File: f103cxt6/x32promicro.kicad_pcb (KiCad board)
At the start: 2 copper layers, 17.8 x 33 mm, 24 parts, among them J1 USB2.0_C_v3, J2 ProMicro-LeftPin-NoGND, J3 ProMicro-RightPin, J4 SWD-MCU_Side-10Pin, SW2 SW_Push, U1 AMS1117-3.3, U2 STM32V103C8T6, Y1 8M

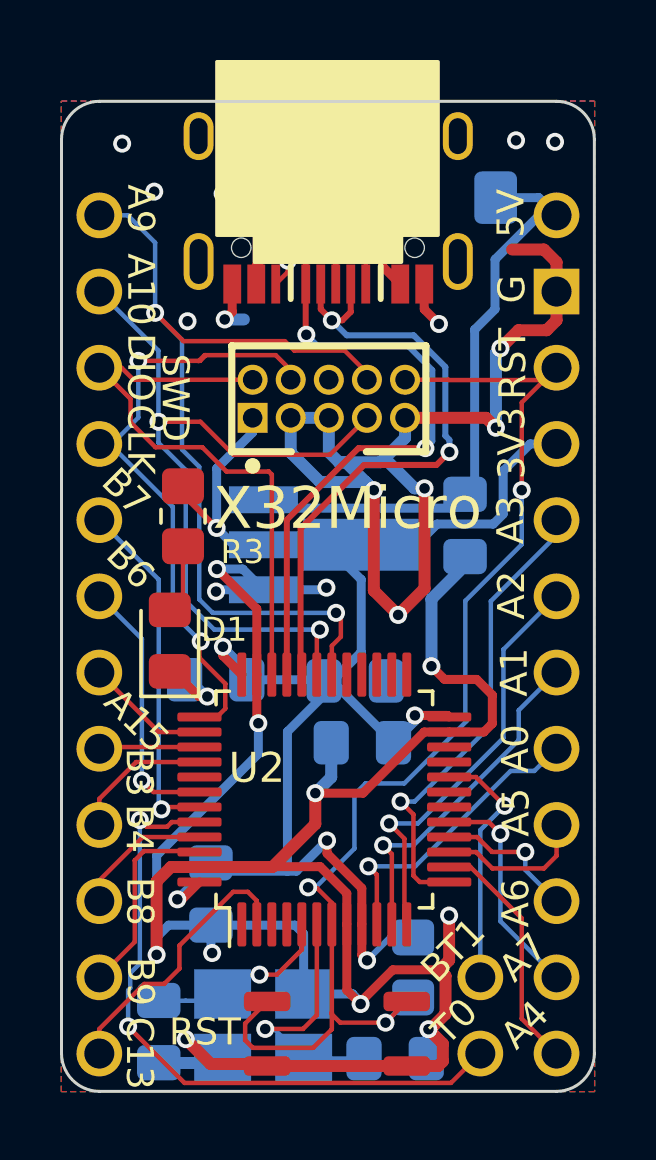
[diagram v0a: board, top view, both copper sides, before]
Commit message: v1.2.0
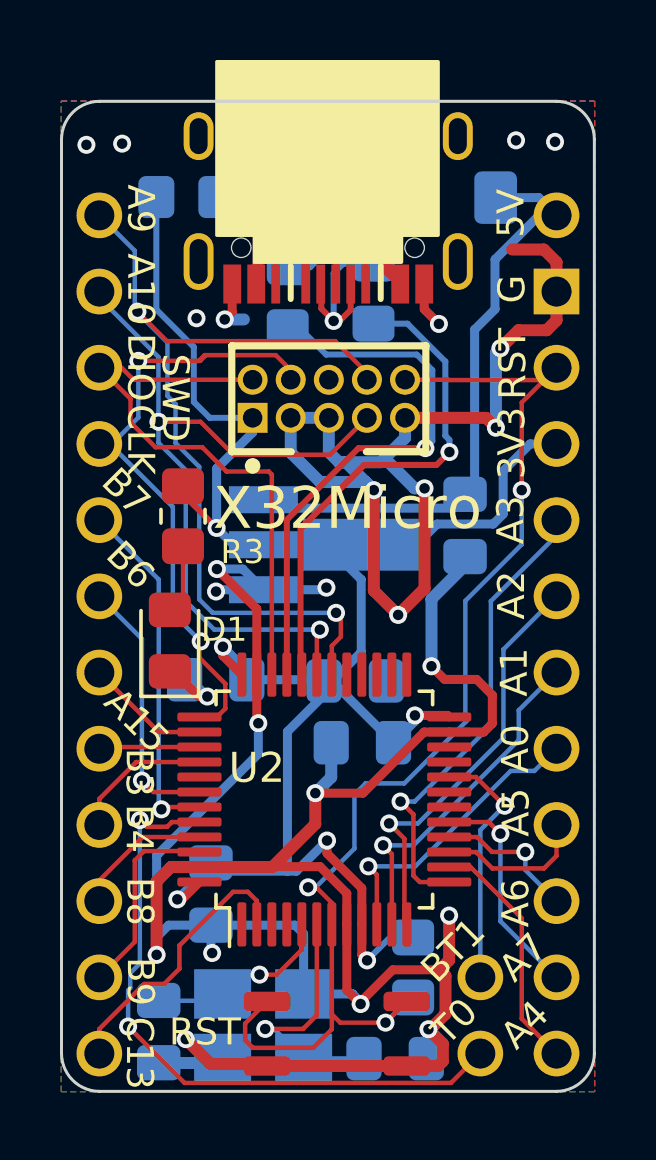
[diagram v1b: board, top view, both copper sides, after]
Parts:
- added R4: 27, $74th:Register_0805_2012, B.Cu at (110.4, 106.4)
- added R5: 27, $74th:Register_0805_2012, B.Cu at (107.5, 106.5)
- added R6: 1.5k, $74th:Register_0805_2012, B.Cu at (104.2, 103.2)
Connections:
- J1 pad 2: /D- -> Net-(J1-D-)
- J1 pad 3: /D+ -> Net-(J1-D+)
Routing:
- net +3V3: track 58.6 -> 68.1 mm
- net Net-(J1-D+): track 0.00 -> 8.21 mm, vias 0 -> 1
- net Net-(J1-D-): track 0.00 -> 6.04 mm, vias 0 -> 1
- net /D+: track 22.8 -> 18.2 mm, vias 2 -> 1
- net /D-: track 21.3 -> 16.9 mm, vias 2 -> 1
- net Net-(J1-VBUS): track 8.84 -> 11.6 mm
- net Net-(J1-CC2): track 4.17 -> 3.29 mm
- net GND: vias 27 -> 28

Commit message: v1.2.0
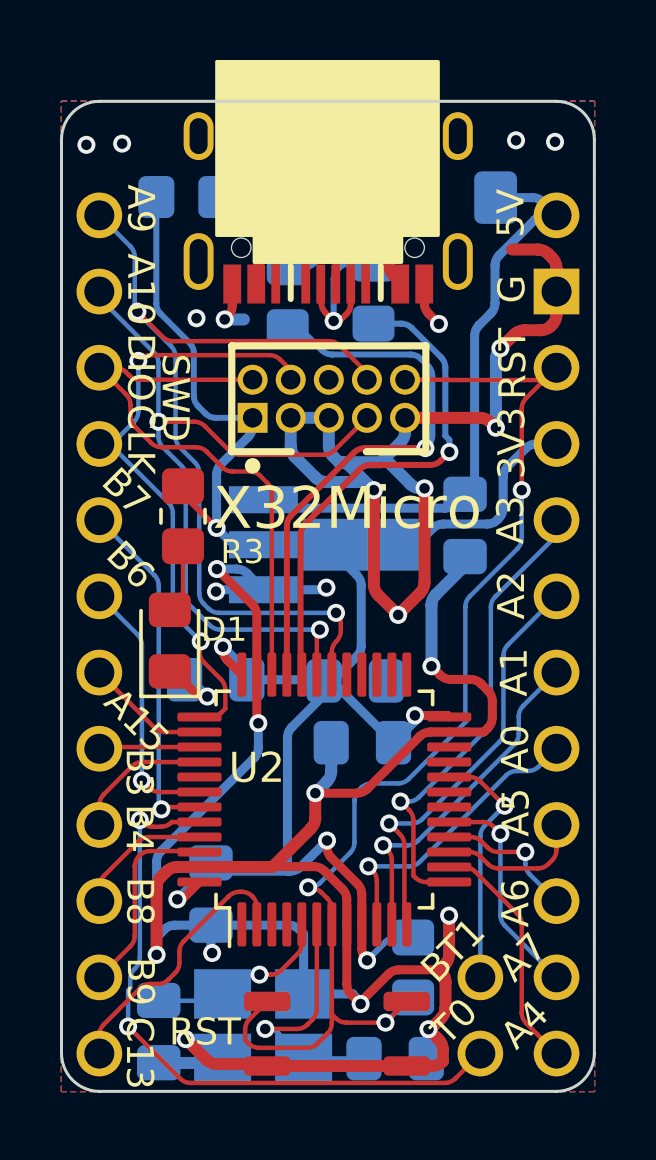
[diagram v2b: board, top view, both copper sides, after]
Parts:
- added REF**: twitter, $74th:twitter, B.Cu at (106.0, 112.4)
- moved G*** 0.33 mm to (104.0, 109.0)
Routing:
- net GND: track 125.4 -> 124.3 mm
- net +3V3: track 68.1 -> 67.5 mm
- net /SWCLK: track 21.3 -> 20.8 mm
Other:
- board text removed: "@74th"
